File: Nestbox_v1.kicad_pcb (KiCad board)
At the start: 2 copper layers, 90 x 23 mm, 81 parts, among them P1 RX/TX, P2 TST/RST, P3 VDD/GND, P4 NFC_PWR_SEL, Q1 SFH 3605, SW1 SMD-BUTTON_2P-3.0X2.5X1.2+0.4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, U1 MSP430FR5969, U2 CR95HF, U3 TPS630250RNC, U4 RN2483, Y1 Crystal, Y2 ABM11-142-27.120MHz

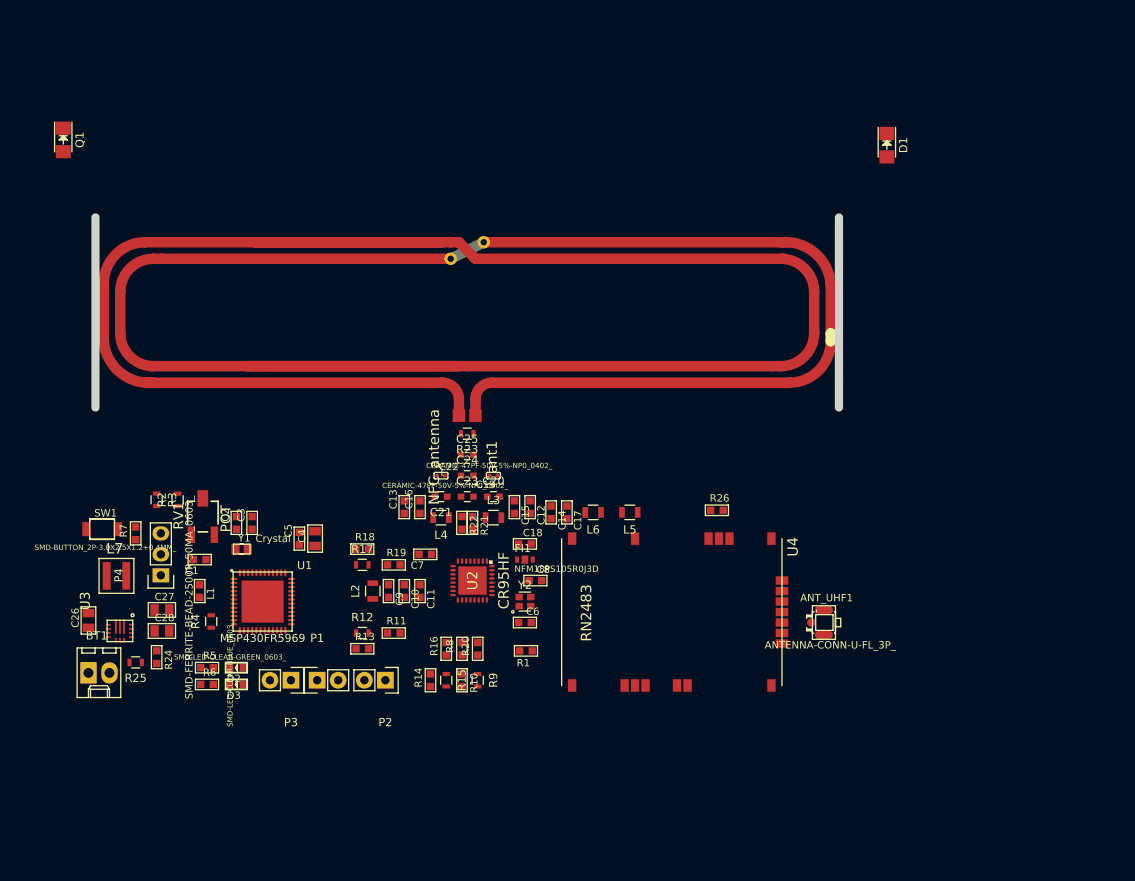
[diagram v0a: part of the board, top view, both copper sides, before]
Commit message: board outline
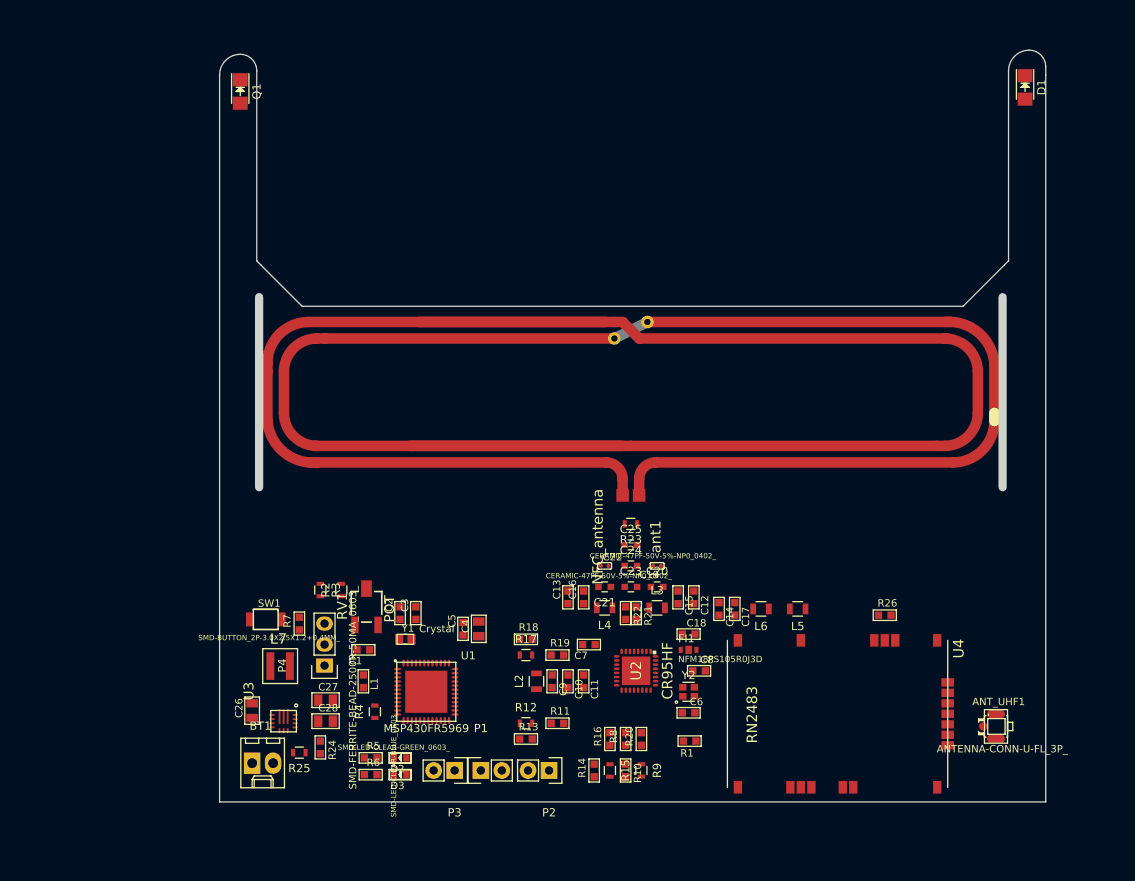
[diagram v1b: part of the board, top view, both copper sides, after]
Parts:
- moved ANT_UHF1 24.3 mm to (190.8, 133.5)
- moved R26 24.0 mm to (177.4, 120.1)
- moved U4 23.5 mm to (158.3, 123.1)
- moved C14 23.4 mm to (157.3, 119.3)
- moved C17 23.4 mm to (159.2, 119.3)
- moved L5 23.4 mm to (166.8, 119.3)
- moved L6 23.4 mm to (162.4, 119.3)
- moved BT1 22.6 mm to (100.8, 138.0)
- moved C10 22.6 mm to (139.0, 128.1)
- moved C11 22.6 mm to (140.9, 128.1)
- moved C6 22.6 mm to (153.6, 131.9)
- moved C9 22.6 mm to (137.1, 128.1)
- moved FI1 22.6 mm to (153.6, 124.2)
- moved L2 22.6 mm to (135.2, 128.1)
- moved L3 22.6 mm to (149.8, 119.2)
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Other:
- board size 90 x 23 mm -> 100 x 91 mm
